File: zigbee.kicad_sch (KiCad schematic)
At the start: 12 parts, among them J13 mrf24j40_tp, J14 mrf24j40_tp, U4 MRF24J40MA

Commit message: Clear remaining KiCad 10-only footprints: SW_Push, kiC, MODULE_MRF24J40MA
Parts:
- U4: footprint MODULE_MRF24J40MA -> (none)
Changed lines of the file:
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@@
 			)
 		)
-		(property "Footprint" "MODULE_MRF24J40MA"
+		(property "Footprint" ""
 			(at 137.16 78.74 0)
 			(hide yes)

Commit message: Extraer footprints de example.kicad_pcb y asignarlos a los esquematicos
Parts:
- U4: footprint (none) -> custom:MODULE_MRF24J40MA
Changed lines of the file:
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@@
 			)
 		)
-		(property "Footprint" ""
+		(property "Footprint" "custom:MODULE_MRF24J40MA"
 			(at 137.16 78.74 0)
 			(hide yes)

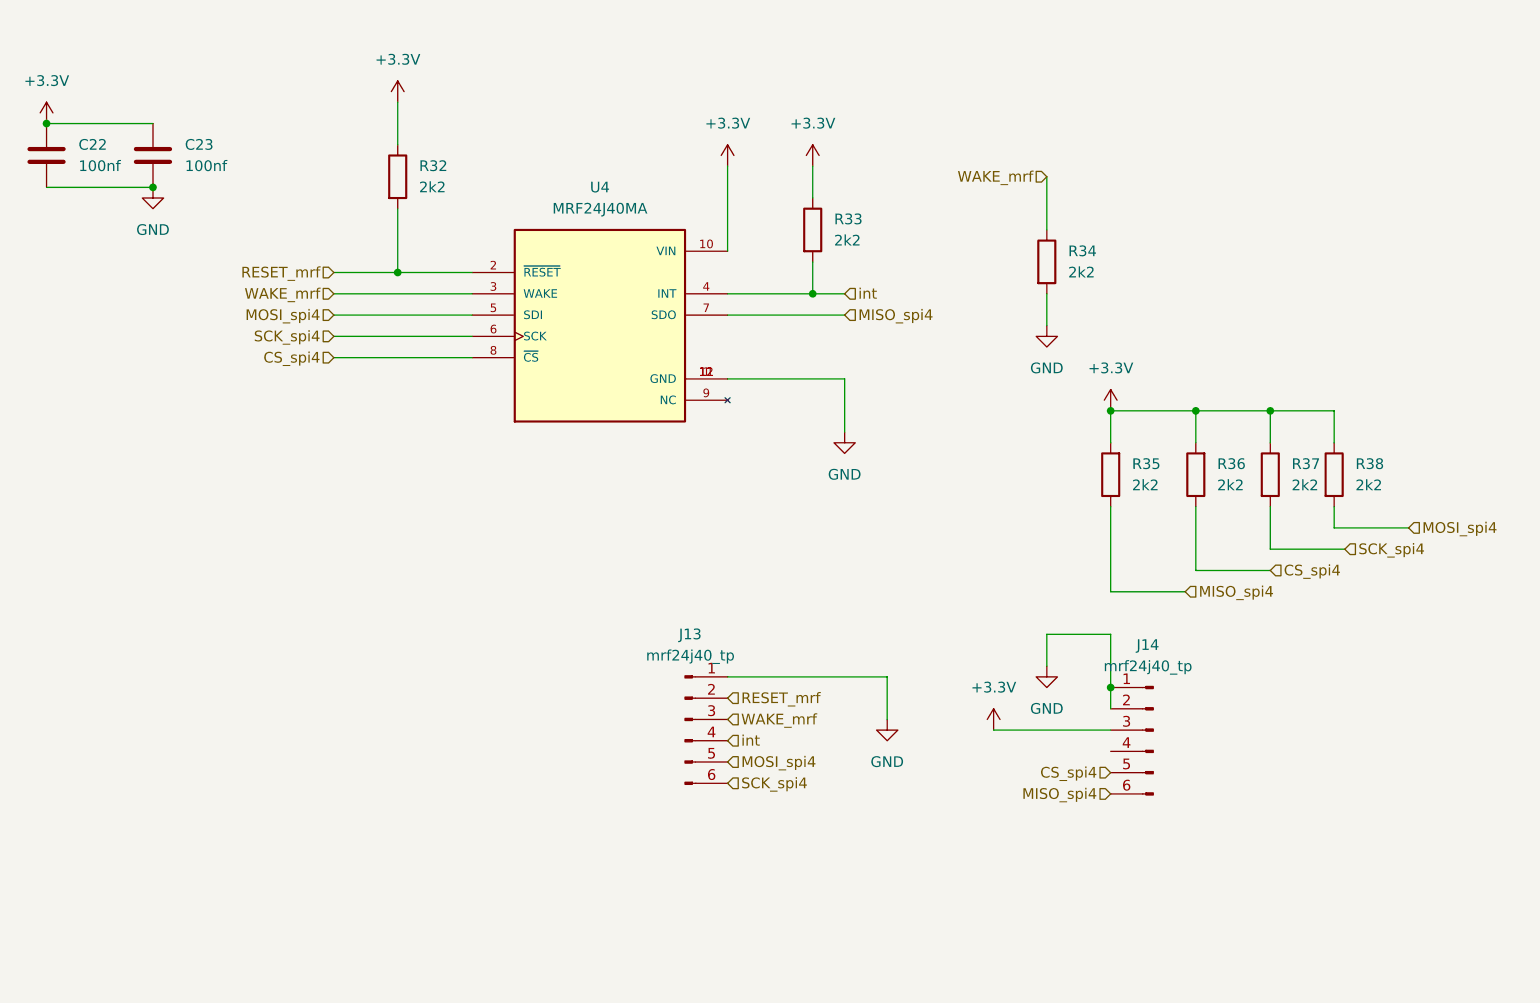
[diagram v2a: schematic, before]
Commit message: CNC Raspberry update
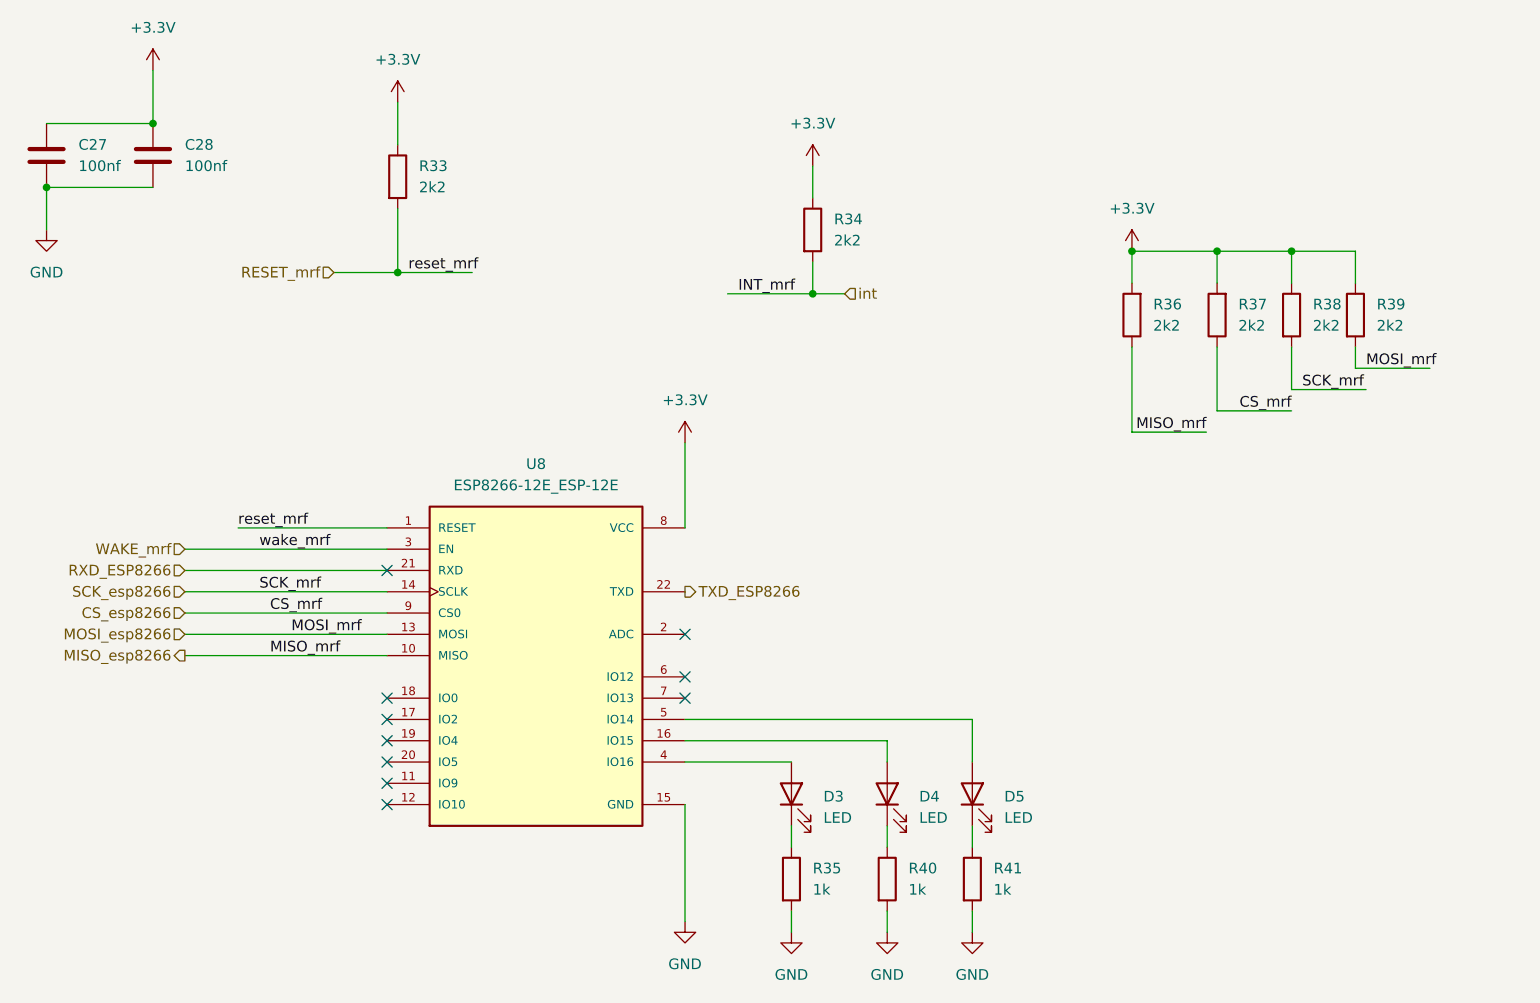
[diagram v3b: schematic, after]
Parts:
- removed J13, J14: mrf24j40_tp, Connector_PinHeader_2.54mm:PinHeader_1x06_P2.54mm_Vertical, symbol Connector:Conn_01x06_Pin
- removed U4: MRF24J40MA, custom:MODULE_MRF24J40MA, symbol RF_ZigBee:MRF24J40MA
- added D3, D4, D5: LED, Diode_SMD:D_0805_2012Metric, symbol Device:LED
- added R40, R41: 1k, Resistor_SMD:R_0805_2012Metric, symbol Device:R
- added U8: ESP8266-12E_ESP-12E, RF_Module:ESP-12E, symbol ESP8266-12E_ESP-12E:ESP8266-12E_ESP-12E
- C27: renamed from C22; footprint Capacitor_SMD:C_0805_2012Metric -> Resistor_SMD:R_0603_1608Metric
- C28: renamed from C23; footprint Capacitor_SMD:C_0805_2012Metric -> Resistor_SMD:R_0603_1608Metric
- R35: renamed from R34; value 2k2 -> 1k; footprint Resistor_SMD:R_0603_1608Metric -> Resistor_SMD:R_0805_2012Metric
- renumbered R32 to R33, R33 to R34, R35 to R36, R36 to R37, R37 to R38, R38 to R39
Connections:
- net +3.3V: now also U8.8 (VCC)
- net GND: now also R40.2, R41.2, U8.15 (GND)
- net RESET_mrf: now also U8.1 (RESET)
- net WAKE_mrf: now also U8.3 (EN); no longer R35.1
- net CS_spi4 renamed CS_esp8266
- net CS_esp8266: now also U8.9 (CS0)
- net MISO_spi4 renamed MISO_esp8266
- net MISO_esp8266: now also U8.10 (MISO)
- net MOSI_spi4 renamed MOSI_esp8266
- net MOSI_esp8266: now also U8.13 (MOSI)
- net SCK_spi4 renamed SCK_esp8266
- net SCK_esp8266: now also U8.14 (SCLK)
- new net: D3.1 (K), R35.1
- new net: D3.2 (A), U8.4 (IO16)
- new net: D4.1 (K), R40.1
- new net: D4.2 (A), U8.16 (IO15)
- new net: D5.2 (A), U8.5 (IO14)
- new net: D5.1 (K), R41.1
- new net RXD_ESP8266: U8.21 (RXD)
- new net TXD_ESP8266: U8.22 (TXD)
- no-connect marks 0 -> 10
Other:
- moved on the sheet: R35, R36, R37, R38, R39
